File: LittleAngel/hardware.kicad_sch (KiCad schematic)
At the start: 16 parts

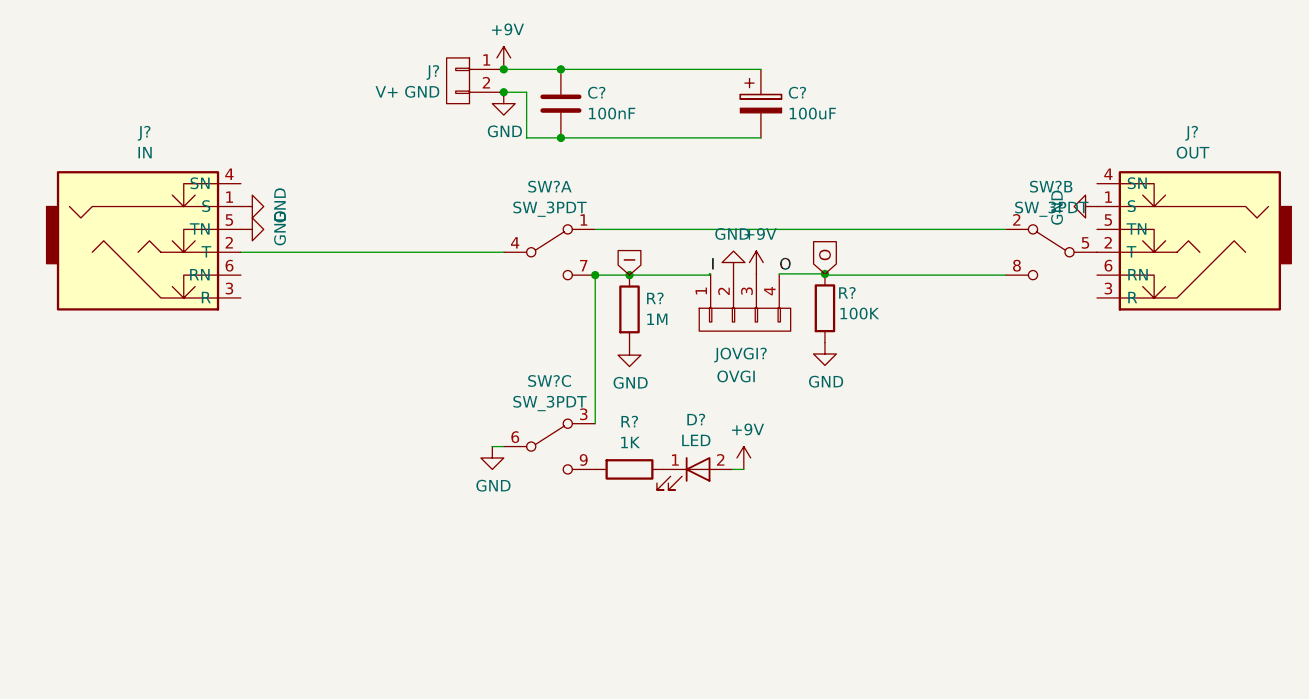
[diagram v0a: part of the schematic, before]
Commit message: WIP
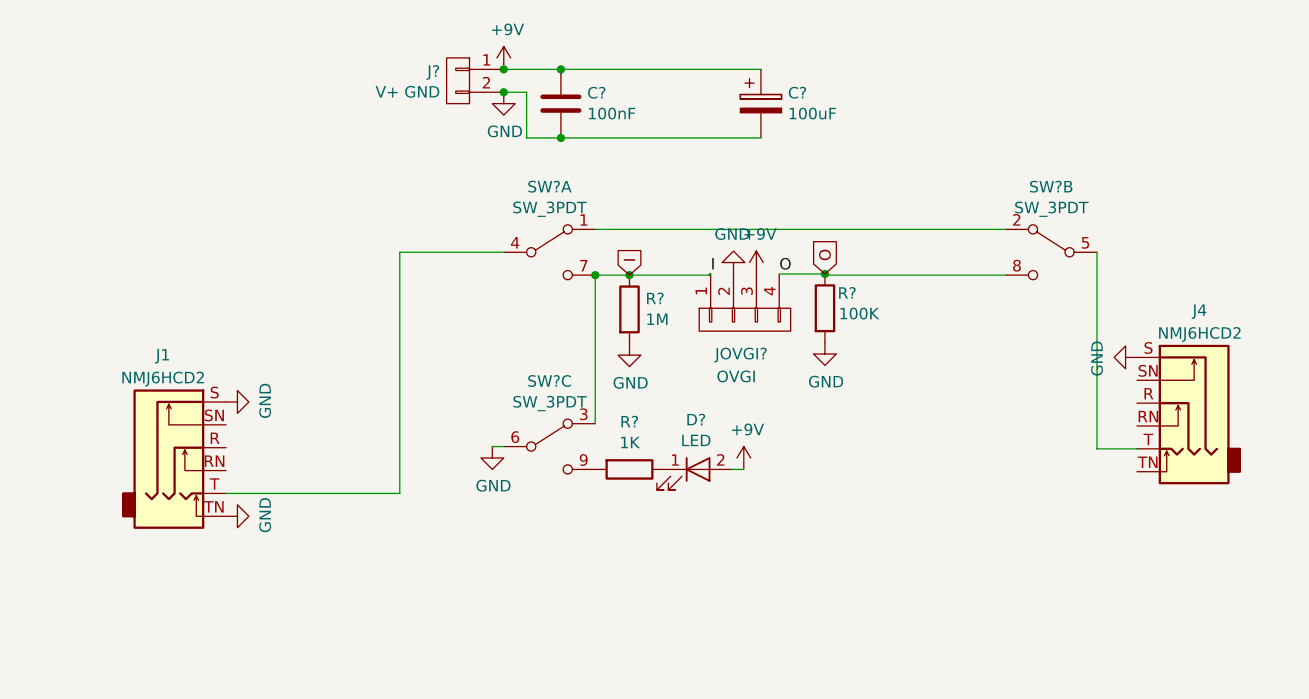
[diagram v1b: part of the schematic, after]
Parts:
- removed J?: OUT, Pedal-Components:Jack_6.35mm_Neutrik_NMJ6HCD2_Horizontal, symbol 1590B-rescue:JACK_TRS_6PINS-conn
- removed J?: IN, Pedal-Components:Jack_6.35mm_Neutrik_NMJ6HCD2_Horizontal, symbol 1590B-rescue:JACK_TRS_6PINS-conn
- added J1, J4: NMJ6HCD2, Connector_Audio:Jack_6.35mm_Neutrik_NMJ6HCD2_Horizontal, symbol Connector_Audio:NMJ6HCD2
- C?: footprint Capacitors_ThroughHole:C_Rect_L7_W3.5_P5 -> Capacitor_SMD:C_0805_2012Metric_Pad1.18x1.45mm_HandSolder
- R? (x3): footprint Resistors_ThroughHole:Resistor_Horizontal_RM7mm -> Resistor_SMD:R_0805_2012Metric_Pad1.20x1.40mm_HandSolder
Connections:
- net GND: now also J1.S, J1.TN, J4.S
- net at SW?.5 (B): now also J4.T
- net at SW?.4 (B): now also J1.T
